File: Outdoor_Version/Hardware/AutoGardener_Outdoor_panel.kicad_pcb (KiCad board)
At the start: 2 copper layers, 94 x 94 mm, 311 parts, among them J1 SWO, J2 Header_1x3, J3 Header_1x3, J4 Header_1x2, Q1 2N7002P.215, Q2 2N7002P.215, U1 STM32L031K6T6, U2 AP2204RB-3.3TRG1

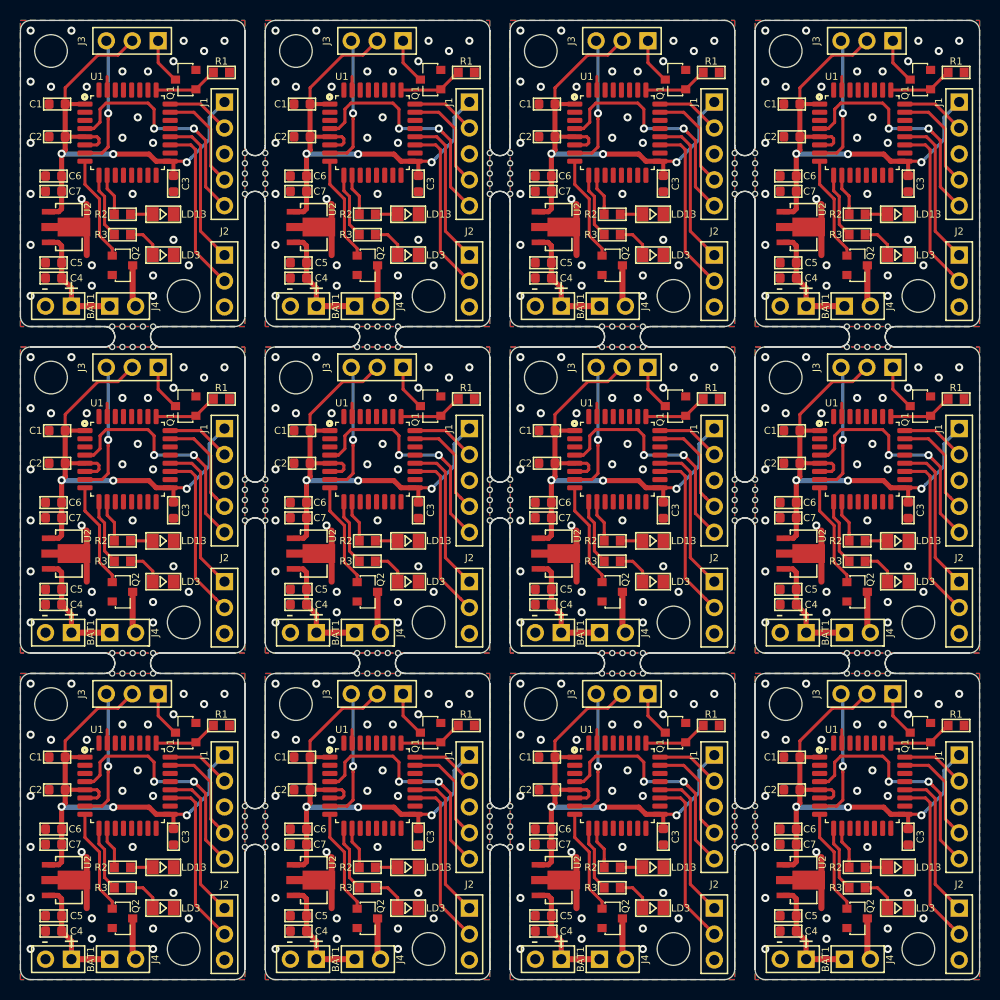
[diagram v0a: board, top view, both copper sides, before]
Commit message: Merging.
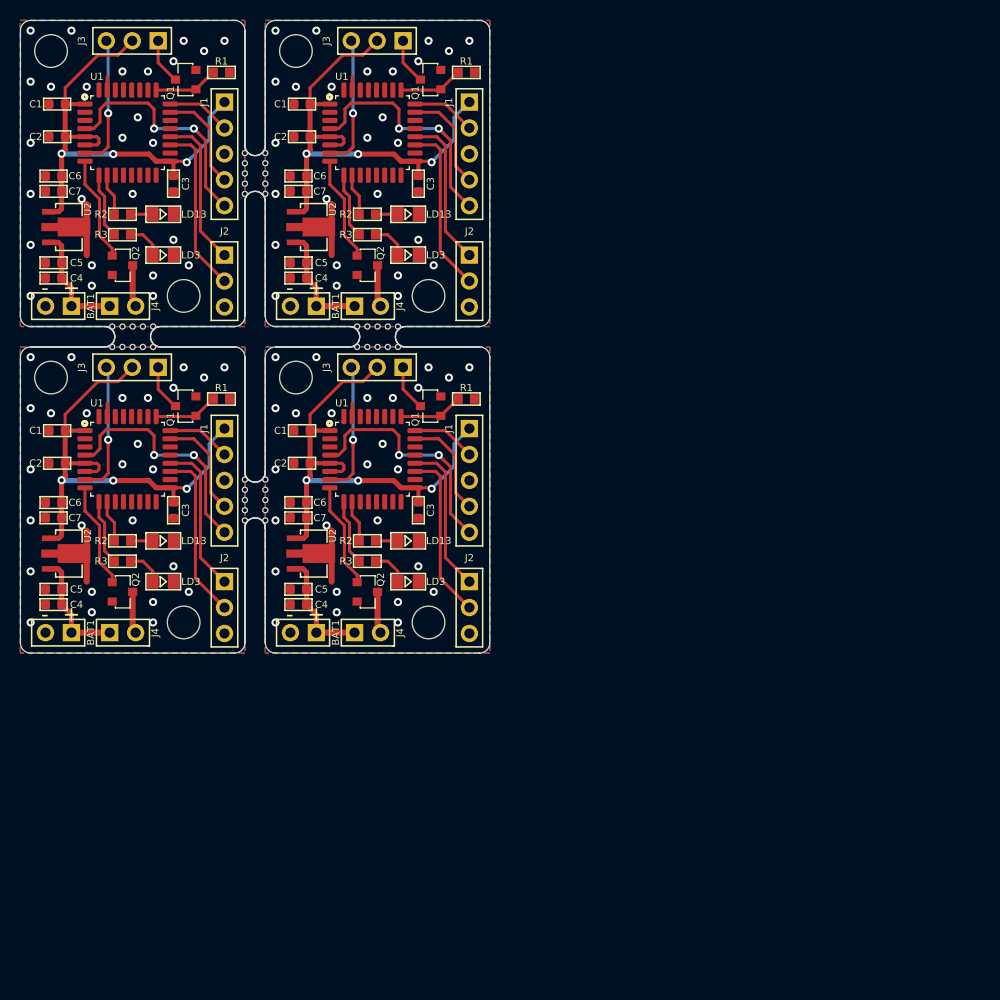
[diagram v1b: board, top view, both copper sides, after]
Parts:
- removed the BAT1 at (233.0, 148.0)
- removed the BAT1 at (209.0, 148.0)
- removed the BAT1 at (185.0, 148.0)
- removed the BAT1 at (233.0, 84.0)
- removed the BAT1 at (257.0, 84.0)
- removed the BAT1 at (233.0, 116.0)
- removed the BAT1 at (257.0, 116.0)
- removed the BAT1 at (257.0, 148.0)
- removed the C1 at (231.6, 128.2)
- removed the C1 at (207.6, 128.2)
- removed the C1 at (183.6, 128.2)
- removed the C1 at (231.6, 64.2)
- removed the C1 at (255.6, 64.2)
- removed the C1 at (231.6, 96.2)
- removed the C1 at (255.6, 96.2)
- removed the C1 at (255.6, 128.2)
- removed the C2 at (231.6, 131.4)
- removed the C2 at (207.6, 131.4)
- removed the C2 at (183.6, 131.4)
- removed the C2 at (231.6, 67.4)
- removed the C2 at (255.6, 67.4)
- removed the C2 at (231.6, 99.4)
- removed the C2 at (255.6, 99.4)
- removed the C2 at (255.6, 131.4)
- removed the C3 at (267.0, 72.0)
- removed the C3 at (243.0, 136.0)
- removed the C3 at (219.0, 136.0)
- removed the C3 at (195.0, 136.0)
- removed the C3 at (243.0, 72.0)
- removed the C3 at (267.0, 104.0)
- removed the C3 at (243.0, 104.0)
- removed the C3 at (267.0, 136.0)
- removed the C4 at (231.2, 145.2)
- removed the C4 at (207.2, 145.2)
- removed the C4 at (183.2, 145.2)
- removed the C4 at (231.2, 81.2)
- removed the C4 at (255.2, 81.2)
- removed the C4 at (231.2, 113.2)
- removed the C4 at (255.2, 113.2)
- removed the C4 at (255.2, 145.2)
- removed the C5 at (231.2, 143.8)
- removed the C5 at (207.2, 143.8)
- removed the C5 at (183.2, 143.8)
- removed the C5 at (231.2, 79.8)
- removed the C5 at (255.2, 79.8)
- removed the C5 at (231.2, 111.8)
- removed the C5 at (255.2, 111.8)
- removed the C5 at (255.2, 143.8)
- removed the C6 at (231.2, 135.2)
- removed the C6 at (207.2, 135.2)
- removed the C6 at (183.2, 135.2)
- removed the C6 at (231.2, 71.2)
- removed the C6 at (255.2, 71.2)
- removed the C6 at (231.2, 103.2)
- removed the C6 at (255.2, 103.2)
- removed the C6 at (255.2, 135.2)
- removed the C7 at (231.2, 136.8)
- removed the C7 at (207.2, 136.8)
- removed the C7 at (183.2, 136.8)
- removed the C7 at (231.2, 72.8)
- removed the C7 at (255.2, 72.8)
- removed the C7 at (231.2, 104.8)
- removed the C7 at (255.2, 104.8)
- removed the C7 at (255.2, 136.8)
- removed the H1 at (231.0, 59.0)
- removed the H1 at (231.0, 123.0)
- removed the H1 at (207.0, 123.0)
- removed the H1 at (183.0, 123.0)
- removed the H1 at (255.0, 59.0)
- removed the H1 at (231.0, 91.0)
- removed the H1 at (255.0, 91.0)
- removed the H1 at (255.0, 123.0)
- removed H111: Mr_Gardener_Logo_Small, Logos:mrg_gardener_08mm
- removed the H2 at (244.0, 83.0)
- removed the H2 at (244.0, 147.0)
- removed the H2 at (220.0, 147.0)
- removed the H2 at (196.0, 147.0)
- removed the H2 at (268.0, 83.0)
- removed the H2 at (244.0, 115.0)
- removed the H2 at (268.0, 115.0)
- removed the H2 at (268.0, 147.0)
- removed the H3 at (263.0, 88.0)
- removed the H3 at (239.0, 88.0)
- removed the H3 at (263.0, 120.0)
- removed the H3 at (239.0, 120.0)
- removed the H3 at (215.0, 120.0)
- removed the H3 at (191.0, 120.0)
- removed the H4 at (239.0, 86.0)
- removed the H4 at (263.0, 86.0)
- removed the H4 at (239.0, 118.0)
- removed the H4 at (263.0, 118.0)
- removed the H4 at (215.0, 118.0)
- removed the H4 at (191.0, 118.0)
- removed the H5 at (226.0, 71.0)
- removed the H5 at (250.0, 71.0)
- removed the H5 at (226.0, 103.0)
- removed the H5 at (250.0, 103.0)
- removed the H5 at (250.0, 135.0)
- removed the H5 at (226.0, 135.0)
- removed the H5 at (202.0, 135.0)
- removed the H6 at (228.0, 71.0)
- removed the H6 at (252.0, 71.0)
- removed the H6 at (228.0, 103.0)
- removed the H6 at (252.0, 103.0)
- removed the H6 at (252.0, 135.0)
- removed the H6 at (228.0, 135.0)
- removed the H6 at (204.0, 135.0)
- removed the J1 at (248.0, 128.0)
- removed the J1 at (224.0, 128.0)
- removed the J1 at (200.0, 128.0)
- removed the J1 at (248.0, 64.0)
- removed the J1 at (272.0, 64.0)
- removed the J1 at (248.0, 96.0)
- removed the J1 at (272.0, 96.0)
- removed the J1 at (272.0, 128.0)
- removed the J2 at (248.0, 143.0)
- removed the J2 at (224.0, 143.0)
- removed the J2 at (200.0, 143.0)
- removed the J2 at (248.0, 79.0)
- removed the J2 at (272.0, 79.0)
- removed the J2 at (248.0, 111.0)
- removed the J2 at (272.0, 111.0)
- removed the J2 at (272.0, 143.0)
- removed the J3 at (241.5, 58.0)
- removed the J3 at (241.5, 122.0)
- removed the J3 at (217.5, 122.0)
- removed the J3 at (193.5, 122.0)
- removed the J3 at (265.5, 58.0)
- removed the J3 at (241.5, 90.0)
- removed the J3 at (265.5, 90.0)
- removed the J3 at (265.5, 122.0)
- removed the J4 at (236.8, 148.0)
- removed the J4 at (212.8, 148.0)
- removed the J4 at (188.8, 148.0)
- removed the J4 at (236.8, 84.0)
- removed the J4 at (260.8, 84.0)
- removed the J4 at (236.8, 116.0)
- removed the J4 at (260.8, 116.0)
- removed the J4 at (260.8, 148.0)
- removed the LD13 at (242.0, 139.0)
- removed the LD13 at (218.0, 139.0)
- removed the LD13 at (194.0, 139.0)
- removed the LD13 at (242.0, 75.0)
- removed the LD13 at (266.0, 75.0)
- removed the LD13 at (242.0, 107.0)
- removed the LD13 at (266.0, 107.0)
- removed the LD13 at (266.0, 139.0)
- removed the LD3 at (242.0, 143.0)
- removed the LD3 at (218.0, 143.0)
- removed the LD3 at (194.0, 143.0)
- removed the LD3 at (242.0, 79.0)
- removed the LD3 at (266.0, 79.0)
- removed the LD3 at (242.0, 111.0)
- removed the LD3 at (266.0, 111.0)
- removed the LD3 at (266.0, 143.0)
- removed the Q1 at (244.2, 125.8)
- removed the Q1 at (220.2, 125.8)
- removed the Q1 at (196.2, 125.8)
- removed the Q1 at (244.2, 61.8)
- removed the Q1 at (268.2, 61.8)
- removed the Q1 at (244.2, 93.8)
- removed the Q1 at (268.2, 93.8)
- removed the Q1 at (268.2, 125.8)
- removed the Q2 at (238.0, 144.0)
- removed the Q2 at (214.0, 144.0)
- removed the Q2 at (190.0, 144.0)
- removed the Q2 at (238.0, 80.0)
- removed the Q2 at (262.0, 80.0)
- removed the Q2 at (238.0, 112.0)
- removed the Q2 at (262.0, 112.0)
- removed the Q2 at (262.0, 144.0)
- removed the R1 at (247.7, 125.1)
- removed the R1 at (223.7, 125.1)
- removed the R1 at (199.7, 125.1)
- removed the R1 at (247.7, 61.1)
- removed the R1 at (271.7, 61.1)
- removed the R1 at (247.7, 93.1)
- removed the R1 at (271.7, 93.1)
- removed the R1 at (271.7, 125.1)
- removed the R2 at (238.0, 75.0)
- removed the R2 at (238.0, 139.0)
- removed the R2 at (214.0, 139.0)
- removed the R2 at (190.0, 139.0)
- removed the R2 at (262.0, 75.0)
- removed the R2 at (238.0, 107.0)
- removed the R2 at (262.0, 107.0)
- removed the R2 at (262.0, 139.0)
- removed the R3 at (238.0, 77.0)
- removed the R3 at (238.0, 141.0)
- removed the R3 at (214.0, 141.0)
- removed the R3 at (190.0, 141.0)
- removed the R3 at (262.0, 77.0)
- removed the R3 at (238.0, 109.0)
- removed the R3 at (262.0, 109.0)
- removed the R3 at (262.0, 141.0)
- removed the U1 at (238.5, 131.0)
- removed the U1 at (214.5, 131.0)
- removed the U1 at (190.5, 131.0)
- removed the U1 at (238.5, 67.0)
- removed the U1 at (262.5, 67.0)
- removed the U1 at (238.5, 99.0)
- removed the U1 at (262.5, 99.0)
- removed the U1 at (262.5, 131.0)
- removed the U2 at (232.8, 140.2)
- removed the U2 at (208.8, 140.2)
- removed the U2 at (184.8, 140.2)
- removed the U2 at (232.8, 76.2)
- removed the U2 at (256.8, 76.2)
- removed the U2 at (232.8, 108.2)
- removed the U2 at (256.8, 108.2)
- removed the U2 at (256.8, 140.2)
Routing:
- net (no net): track 2168.5 -> 788.6 mm, vias 352 -> 128
- net VCC: track 50.9 -> 0.00 mm, vias 3 -> 0
- net /NRST: track 23.4 -> 0.00 mm, vias 2 -> 0
- net /UART_TX: track 16.7 -> 0.00 mm
- net /UART_RX: track 15.1 -> 0.00 mm
- net /ADC_SOIL1: track 13.0 -> 0.00 mm, vias 1 -> 0
- net +5V: track 11.5 -> 0.00 mm
- net /OUT1: track 10.4 -> 0.00 mm
- net /SWDIO: track 10.2 -> 0.00 mm
- net GND: track 8.11 -> 0.00 mm, vias 26 -> 0
- net /LED1: track 6.75 -> 0.00 mm
- net /SENS_ENA: track 6.33 -> 0.00 mm
- net /SWCLK: track 6.29 -> 0.00 mm
- net Net-(J3-Pad1): track 4.53 -> 0.00 mm
- net /BAT_LO: track 4.12 -> 0.00 mm
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- removed copper zone on B.Cu, net GND
- removed copper zone on F.Cu, net GND
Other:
- board size 94 x 94 mm -> 46 x 62 mm
